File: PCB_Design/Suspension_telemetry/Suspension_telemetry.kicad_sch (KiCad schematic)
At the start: 23 parts, among them J11 530480310, J12 530480410, J2 Conn_01x03_Pin, J3 112J-TDAR-R01, J4 Conn_02x04_Top_Bottom, J6 Conn_01x08_Socket, J7 530480510, J8 530480310, J9 530480410, U5 USBLC6-2SC6

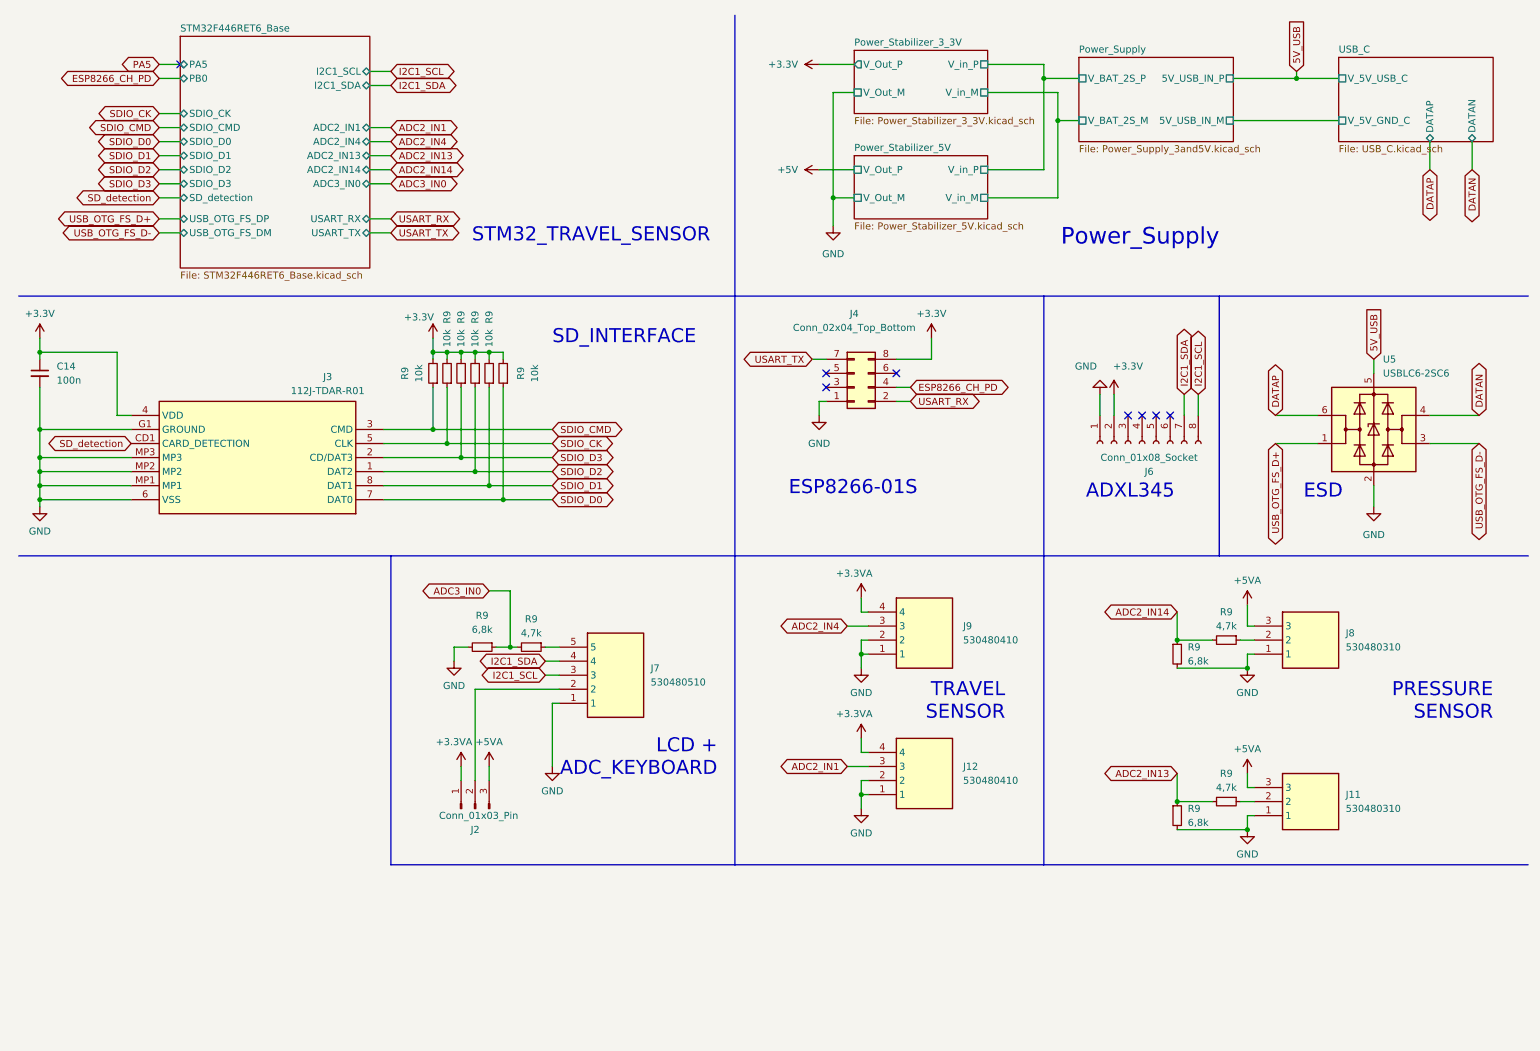
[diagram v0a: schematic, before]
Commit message: pcv v2 finished
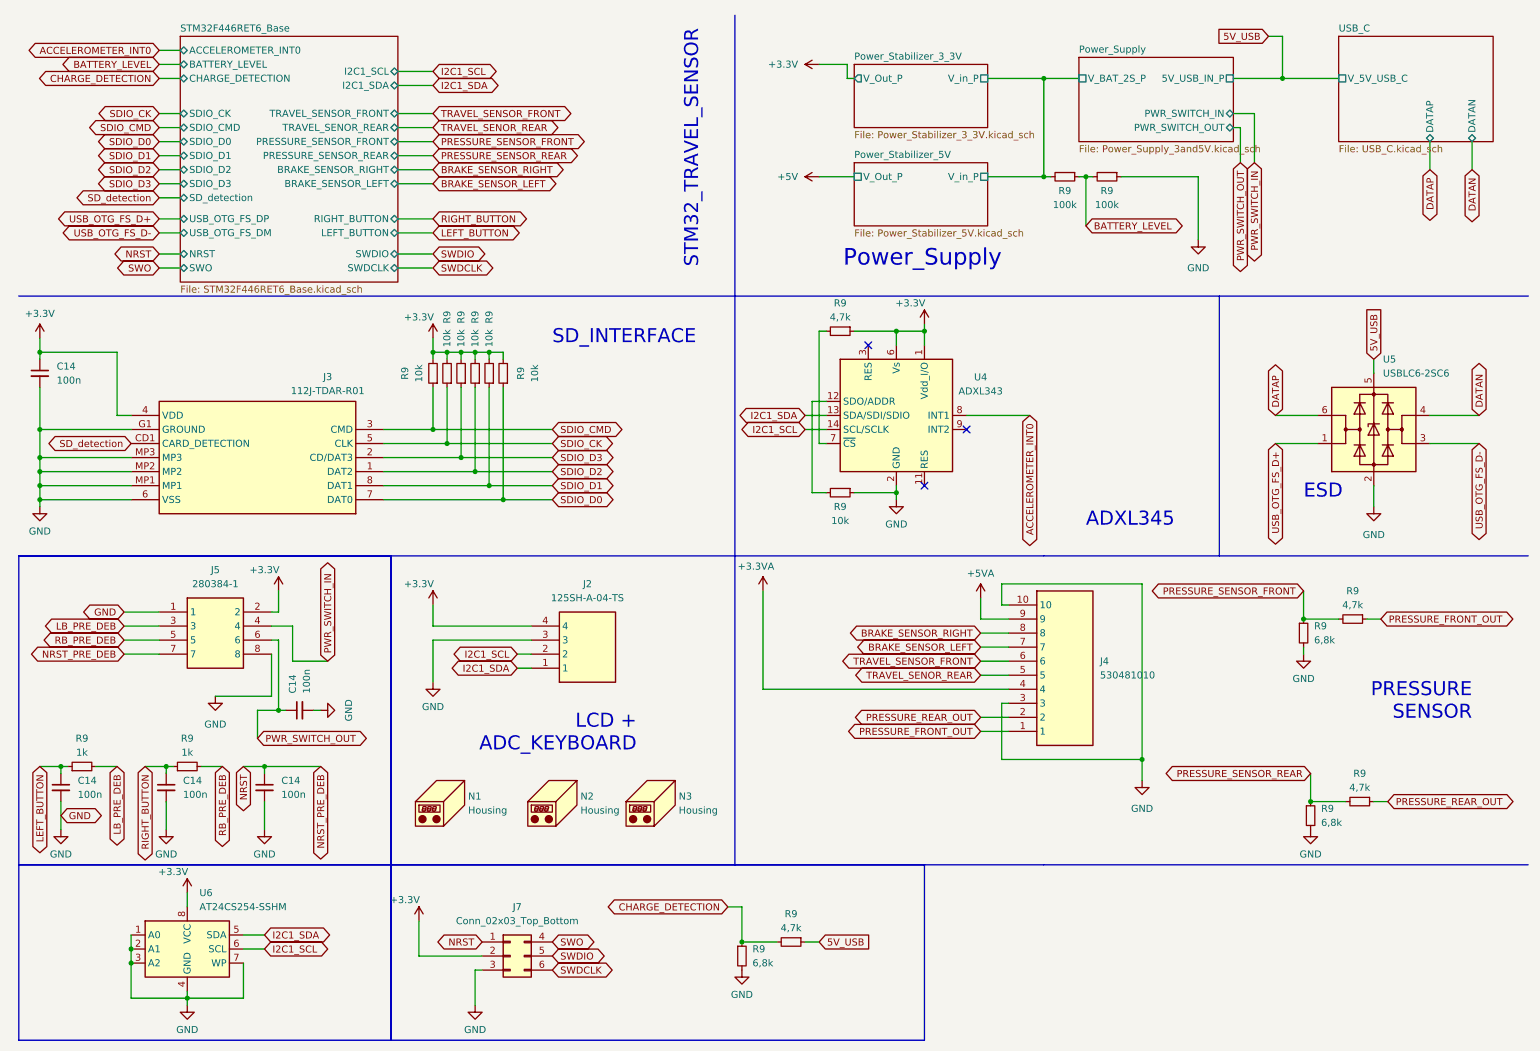
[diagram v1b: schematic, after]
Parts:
- removed J11, J8: 530480310, molex_conn:530480310, symbol 530480310:530480310
- removed J12, J9: 530480410, molex_conn:530480410, symbol 530480410:530480410
- removed J2: Conn_01x03_Pin, Connector_PinHeader_1.27mm:PinHeader_1x03_P1.27mm_Vertical, symbol Connector:Conn_01x03_Pin
- removed J4: Conn_02x04_Top_Bottom, Connector_PinSocket_2.54mm:PinSocket_2x04_P2.54mm_Vertical, symbol connector_my_2x4:Conn_02x04_Top_Bottom_v2
- removed J6: Conn_01x08_Socket, Connector_PinSocket_2.54mm:PinSocket_1x08_P2.54mm_Vertical, symbol Connector:Conn_01x08_Socket
- removed J7: 530480510, molex_conn:530480510, symbol 530480510:530480510
- removed R9 (x2): 6,8k, Resistor_SMD:R_0603_1608Metric_Pad0.98x0.95mm_HandSolder, symbol Device:R_Small
- removed R9 (x2): 4,7k, Resistor_SMD:R_0603_1608Metric_Pad0.98x0.95mm_HandSolder, symbol Device:R_Small
- added C14 (x4): 100n, Capacitor_SMD:C_0603_1608Metric_Pad1.08x0.95mm_HandSolder, symbol Device:C_Small
- added J2: 125SH-A-04-TS, molex_conn:125SHA04TS, symbol MOLEX_4:125SH-A-04-TS
- added J4: 530481010, 530481010, symbol MOLEX_10_pin:530481010
- added J5: 280384-1, BUTTON_CONN:2803841, symbol BUTTON_CONN:280384-1
- added J7: Conn_02x03_Top_Bottom, Connector_PinHeader_2.54mm:PinHeader_2x03_P2.54mm_Vertical, symbol Connector_Generic:Conn_02x03_Top_Bottom
- added N1, N2, N3: Housing, Symbol:CE-Logo_8.5x6mm_SilkScreen, symbol Mechanical:Housing
- added R9 (x2): 6,8k, Resistor_SMD:R_0603_1608Metric_Pad0.98x0.95mm_HandSolder, symbol Device:R_Small
- added R9 (x2): 1k, Resistor_SMD:R_0603_1608Metric_Pad0.98x0.95mm_HandSolder, symbol Device:R_Small
- added R9 (x3): 4,7k, Resistor_SMD:R_0603_1608Metric_Pad0.98x0.95mm_HandSolder, symbol Device:R_Small
- added R9 (x2): 100k, Resistor_SMD:R_0603_1608Metric_Pad0.98x0.95mm_HandSolder, symbol Device:R_Small
- added R9: 10k, Resistor_SMD:R_0603_1608Metric_Pad0.98x0.95mm_HandSolder, symbol Device:R_Small
- added U4: ADXL343, Package_LGA:LGA-14_3x5mm_P0.8mm_LayoutBorder1x6y, symbol Sensor_Motion:ADXL343
- added U6: AT24CS254-SSHM, Package_SO:SOIC-8_3.9x4.9mm_P1.27mm, symbol Memory_EEPROM:AT24CS64-SSHM
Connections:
- net +3.3V: now also J2.4, J5.2, J7.2 (Pin_2), R9.1, U4.1 (Vdd_I/O), U4.6 (Vs), U6.8 (VCC)
- net +3.3VA: now also J4.4
- net +5VA: now also J4.9
- net 5V_USB: now also R9.1
- net GND: now also C14.2, C14.2, C14.2, C14.2, J2.3, J4.10, J4.3, J5.1, J5.8, J7.3 (Pin_3), R9.1, R9.1, R9.2, R9.2, U4.2 (GND), U4.4 (GND), U4.5 (GND), U6.1 (A0), U6.2 (A1), U6.3 (A2), U6.4 (GND), U6.7 (WP)
- net I2C1_SCL: now also J2.2, U4.14 (SCL/SCLK), U6.6 (SCL)
- net I2C1_SDA: now also J2.1, U4.13 (SDA/SDI/SDIO), U6.5 (SDA)
- net Power_Stabilizer_3_3V/V_in_P: now also R9.2
- net PRESSURE_REAR_OUT: now reaches R9.1
- net PRESSURE_REAR_OUT: now also J4.2
- net ADC2_IN14 renamed PRESSURE_SENSOR_REAR
- new net: R9.2, U4.7 (~{CS})
- new net: R9.2, U4.12 (SDO/ADDR)
- new net ACCELEROMETER_INT0: U4.8 (INT1)
- new net BATTERY_LEVEL: R9.1, R9.2
- new net BRAKE_SENSOR_LEFT: J4.7
- new net BRAKE_SENSOR_RIGHT: J4.8
- new net CHARGE_DETECTION: R9.1, R9.2
- new net LB_PRE_DEB: J5.3, R9.2
- new net LEFT_BUTTON: C14.1, R9.1
- new net NRST: C14.1, J5.7, J7.1 (Pin_1)
- new net PRESSURE_FRONT_OUT: J4.1, R9.1
- new net PRESSURE_SENSOR_FRONT: R9.1, R9.2
- new net PWR_SWITCH_IN: J5.4
- new net PWR_SWITCH_OUT: C14.1, J5.6
- new net RB_PRE_DEB: J5.5, R9.2
- new net RIGHT_BUTTON: C14.1, R9.1
- new net SWDCLK: J7.6 (Pin_6)
- new net SWDIO: J7.5 (Pin_5)
- new net SWO: J7.4 (Pin_4)
- new net TRAVEL_SENOR_REAR: J4.5
- new net TRAVEL_SENSOR_FRONT: J4.6
- no-connect marks 8 -> 3
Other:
- sheet Power_Stabilizer_3_3V ports: added none; removed V_Out_M, V_in_M
- sheet Power_Stabilizer_5V ports: added none; removed V_Out_M, V_in_M
- sheet Power_Supply ports: added PWR_SWITCH_IN, PWR_SWITCH_OUT; removed 5V_USB_IN_M, V_BAT_2S_M
- sheet STM32F446RET6_Base ports: added ACCELEROMETER_INT0, BATTERY_LEVEL, BRAKE_SENSOR_LEFT, BRAKE_SENSOR_RIGHT, CHARGE_DETECTION, LEFT_BUTTON, NRST, PRESSURE_SENSOR_FRONT, PRESSURE_SENSOR_REAR, RIGHT_BUTTON, SWDCLK, SWDIO, SWO, TRAVEL_SENOR_REAR, TRAVEL_SENSOR_FRONT; removed ADC2_IN1, ADC2_IN13, ADC2_IN14, ADC2_IN4, ADC3_IN0, PA5, PB0, USART_RX, USART_TX
- sheet USB_C ports: added none; removed V_5V_GND_C
- note removed: "ESP8266-01S"
- note removed: "TRAVEL SENSOR"
- moved on the sheet: R9
